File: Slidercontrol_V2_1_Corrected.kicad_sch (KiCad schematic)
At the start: 9 parts, among them J1 Jack-DC, J2 AudioJack3, J3 AudioPlug3, J4 N3 Canon Camera Connector, U1 4N33

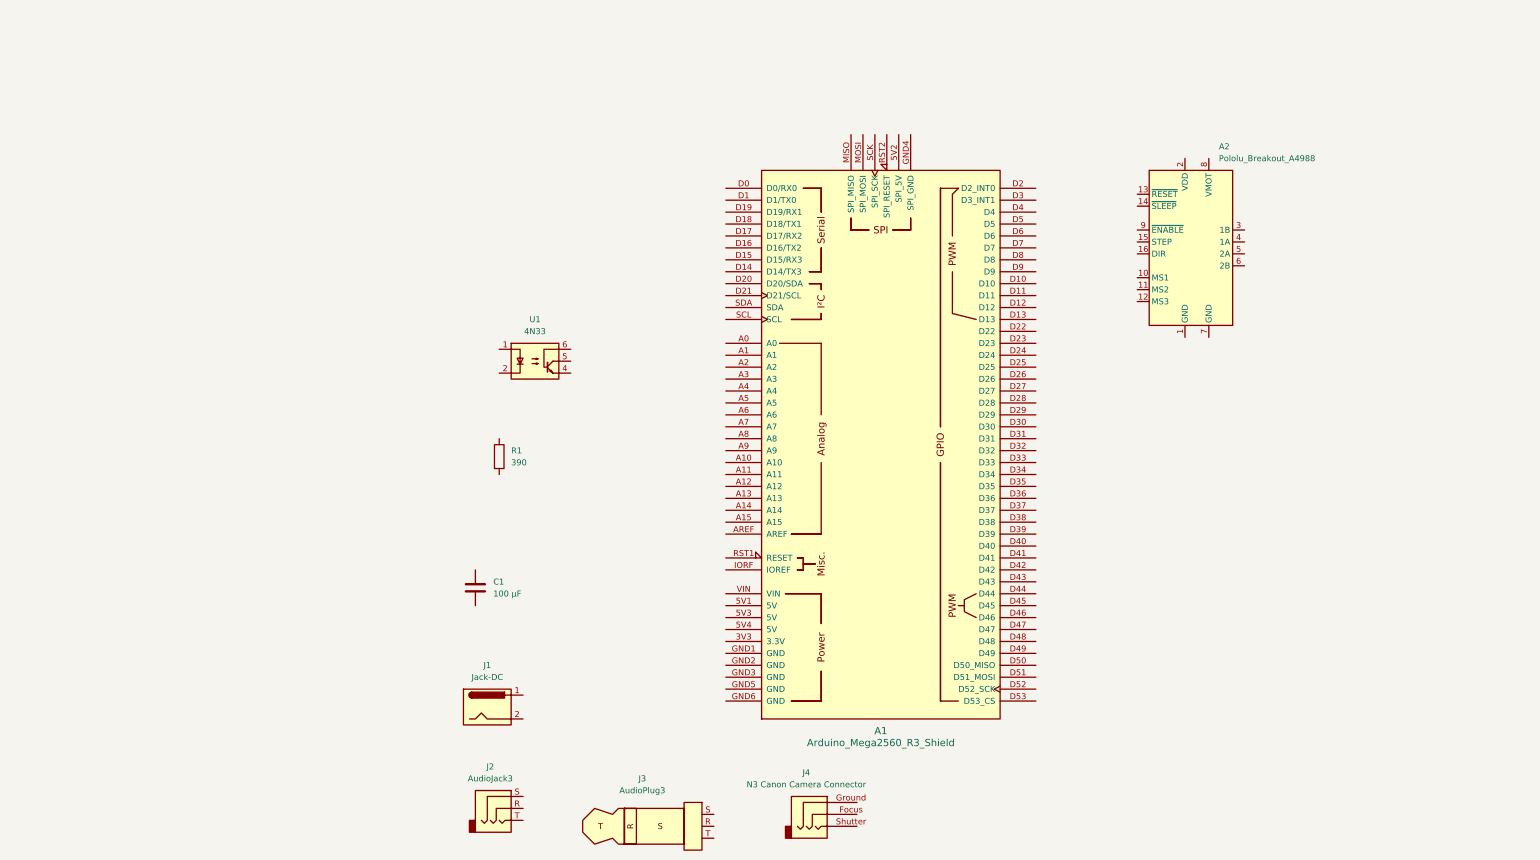
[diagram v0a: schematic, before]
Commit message: Update
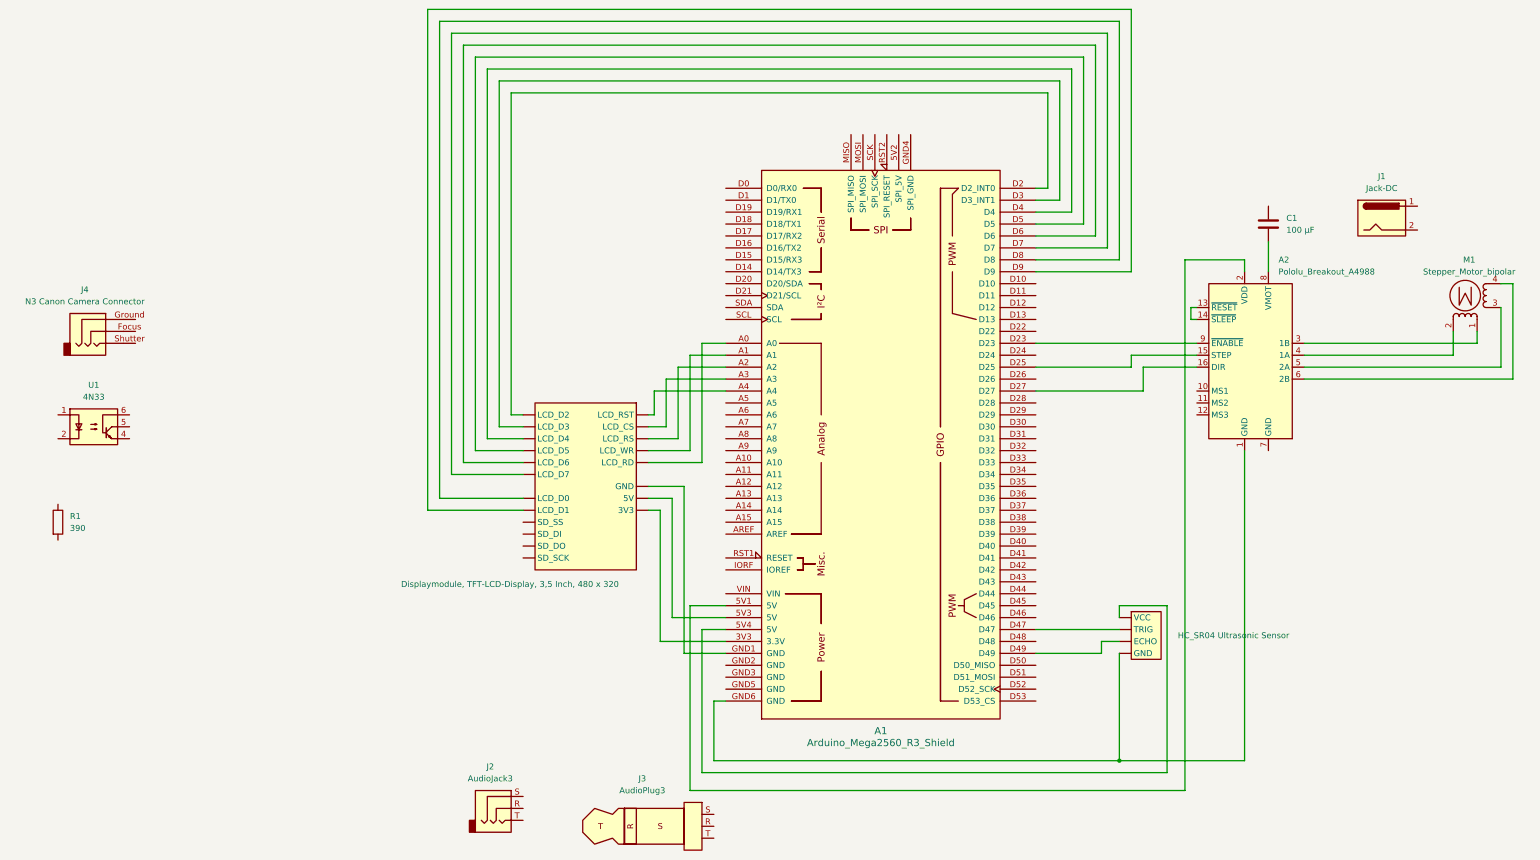
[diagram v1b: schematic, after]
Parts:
- added M1: Stepper_Motor_bipolar, symbol Motor:Stepper_Motor_bipolar
- added U3: HC_SR04 Ultrasonic Sensor, symbol mySymbols:HC_SR04 Ultrasonic Sensor
- added u2: Displaymodule, TFT-LCD-Display, 3,5 Inch, 480 x 3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, symbol mySymbols:Displaymodule,TFT-LCD-Display, 3,5 Inch (8,9cm), 480x320
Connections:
- net at A1.3V3 (3.3V): now also u2. (SD_SCK)
- net at A1.5V1 (5V): now also A2.2 (VDD)
- net at A1.5V3 (5V): now also u2. (SD_SCK)
- net at A1.5V4 (5V): now also U3. (GND)
- net at A1.A0: now also u2. (SD_SCK)
- net at A1.A1: now also u2. (SD_SCK)
- net at A1.A2: now also u2. (SD_SCK)
- net at A1.A3: now also u2. (SD_SCK)
- net at A1.A4: now also u2. (SD_SCK)
- net at A1.D2 (D2_INT0): now also u2. (SD_SCK)
- net at A1.D23: now also A2.9 (~{ENABLE})
- net at A1.D25: now also A2.15 (STEP)
- net at A1.D27: now also A2.16 (DIR)
- net at A1.D3 (D3_INT1): now also u2. (SD_SCK)
- net at A1.D4: now also u2. (SD_SCK)
- net at A1.D47: now also U3. (GND)
- net at A1.D49: now also U3. (GND)
- net at A1.D5: now also u2. (SD_SCK)
- net at A1.D6: now also u2. (SD_SCK)
- net at A1.D7: now also u2. (SD_SCK)
- net at A1.D8: now also u2. (SD_SCK)
- net at A1.D9: now also u2. (SD_SCK)
- net at A1.GND1 (GND): now also u2. (SD_SCK)
- net at A1.GND6 (GND): now also A2.1 (GND), U3. (GND)
- net at C1.2: now also A2.8 (VMOT)
- net at A2.13 (~{RESET}): now also A2.14 (~{SLEEP})
- net at A2.3 (1B): now also M1.1
- net at A2.4 (1A): now also M1.2 (-)
- net at A2.5 (2A): now also M1.3
- net at A2.6 (2B): now also M1.4
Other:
- moved on the sheet: A2, C1, J1, J4, R1, U1
